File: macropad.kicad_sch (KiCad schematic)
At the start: 64 parts, among them J1 USB_C_Receptacle_USB2.0, J3 Conn_01x03, J6 Conn_01x04_Pin, J7 Conn_01x02_Pin, J9 Conn_01x02_Pin, SW1 SW_Push, SW3 SW_Push, SW4 SW_Push, SW5 SW_Push, SW6 RotaryEncoder_Switch, SW7 SW_Push, SW8 SW_Push, SW9 RotaryEncoder_Switch, U1 RP2040, U2 W25Q16JVUXIQ, U3 MIC5504-3.3YM5, U6 SN74LVC1T45DRL, U7 USBLC6-2P6, Y1 Crystal_GND24

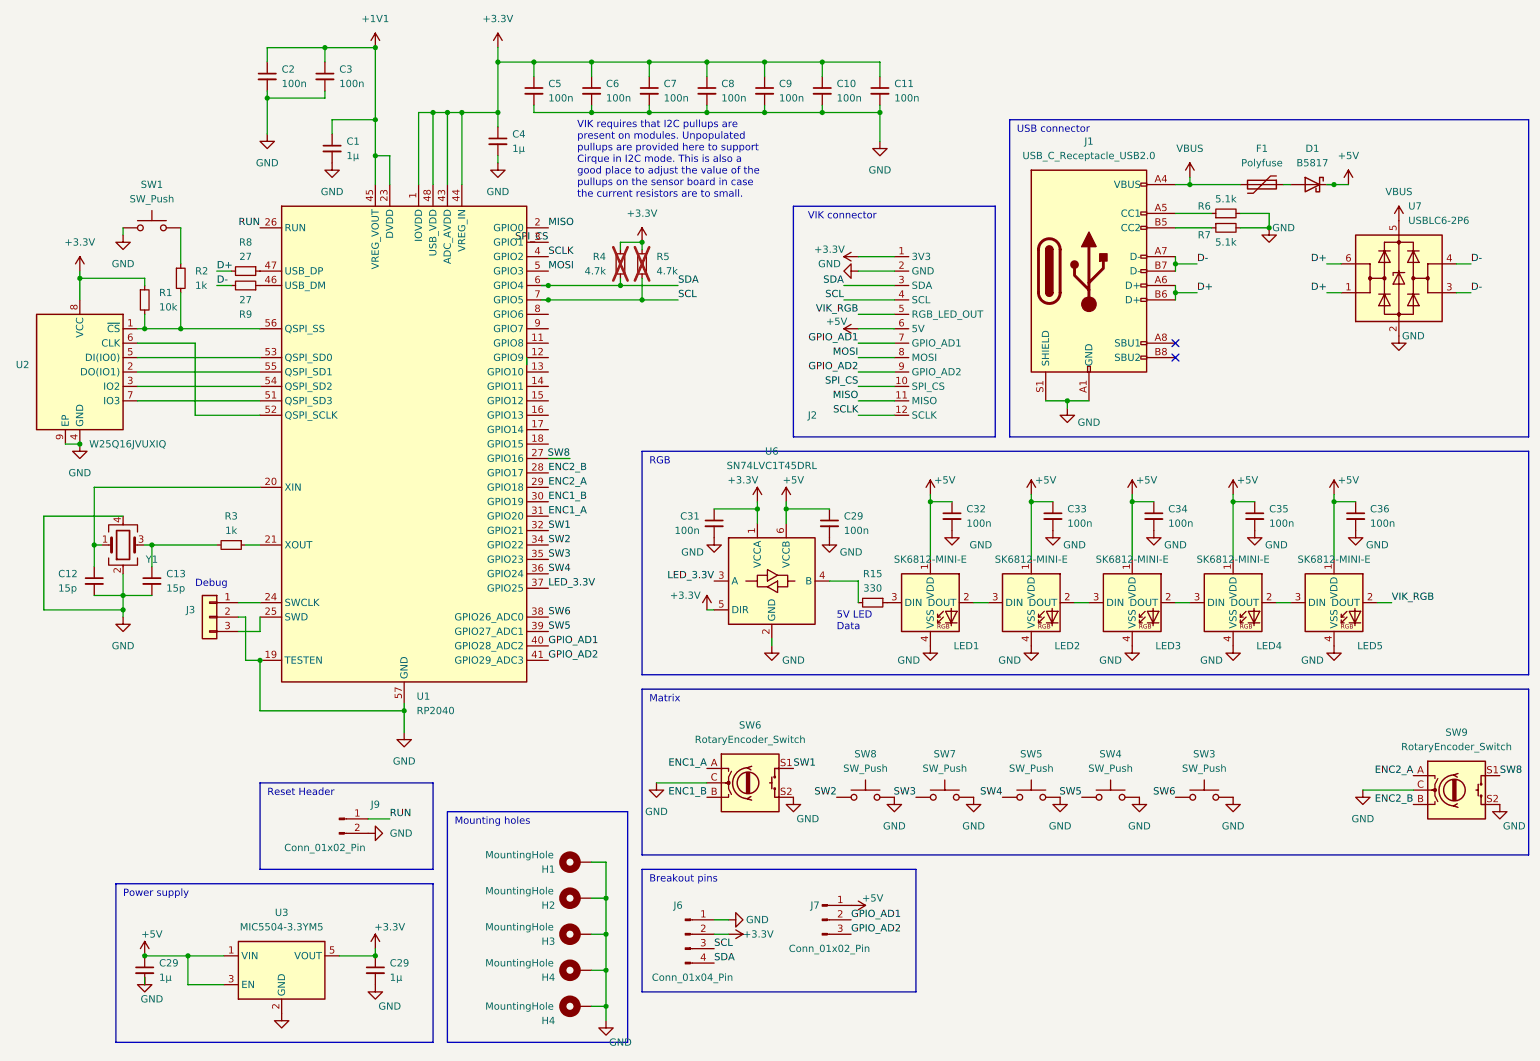
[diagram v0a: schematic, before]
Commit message: Minor tweaks
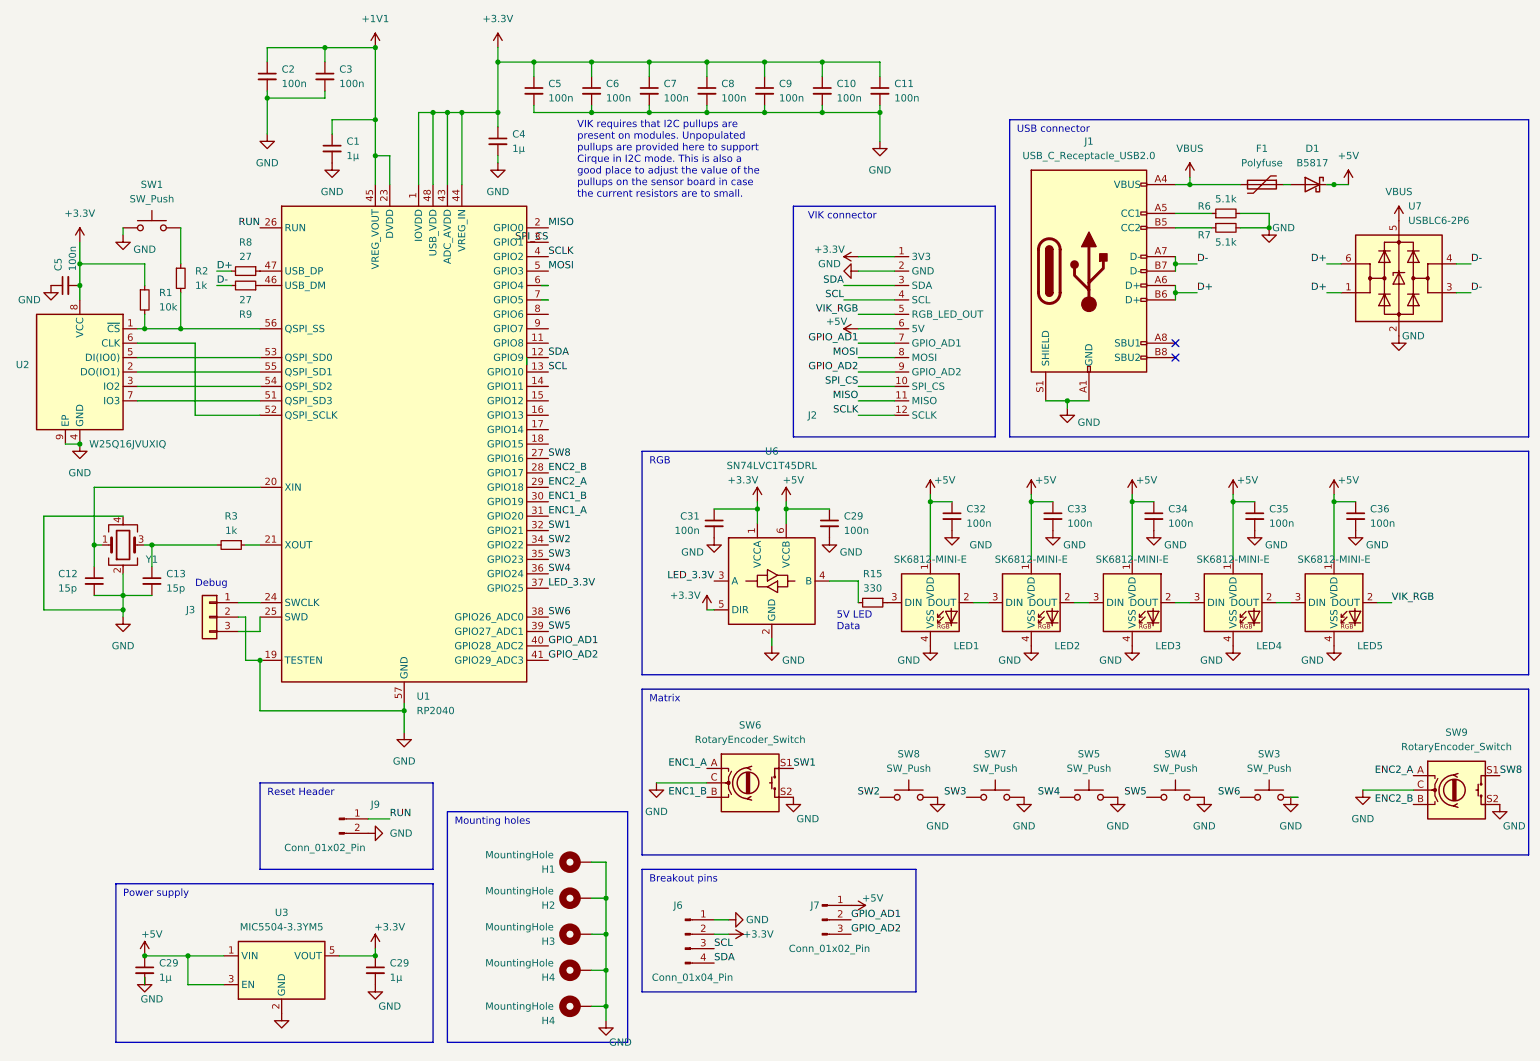
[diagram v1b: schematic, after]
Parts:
- removed R4, R5: 4.7k, Resistor_SMD:R_1206_3216Metric_Pad1.30x1.75mm_HandSolder, symbol Device:R_Small
- added C5: 100n, Capacitor_SMD:C_0402_1005Metric, symbol Device:C_Small
- C29: LCSC C1525 -> C52923
- R15: LCSC (none) -> C25104
- SW1: LCSC C5333465 -> C221821
- SW6: LCSC C5333465 -> (none)
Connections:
- net +3.3V: now also C5.2
- net GND: now also C5.1
- net SCL: now also U1.13 (GPIO10); no longer U1.7 (GPIO5)
- net SDA: now also U1.12 (GPIO9); no longer U1.6 (GPIO4)
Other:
- moved on the sheet: SW3, SW4, SW5, SW7, SW8
